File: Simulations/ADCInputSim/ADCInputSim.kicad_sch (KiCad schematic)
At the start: 8 parts, among them U1 ${SIM.PARAMS}

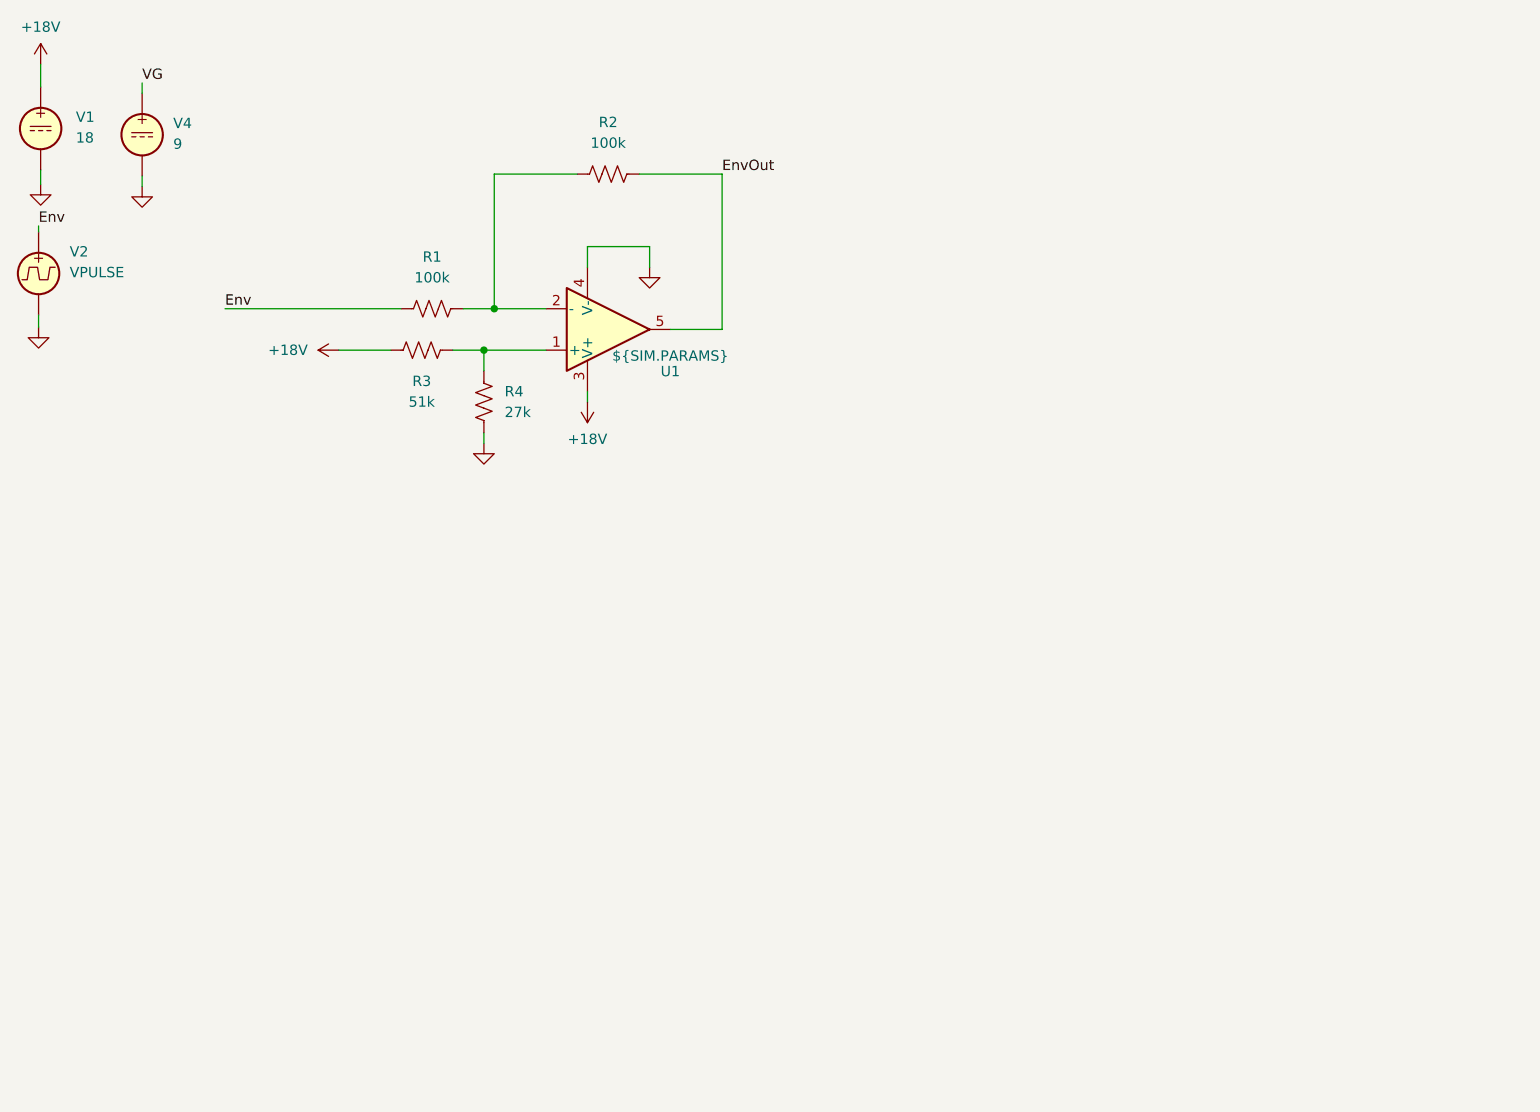
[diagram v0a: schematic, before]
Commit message: ADC driver dialed in
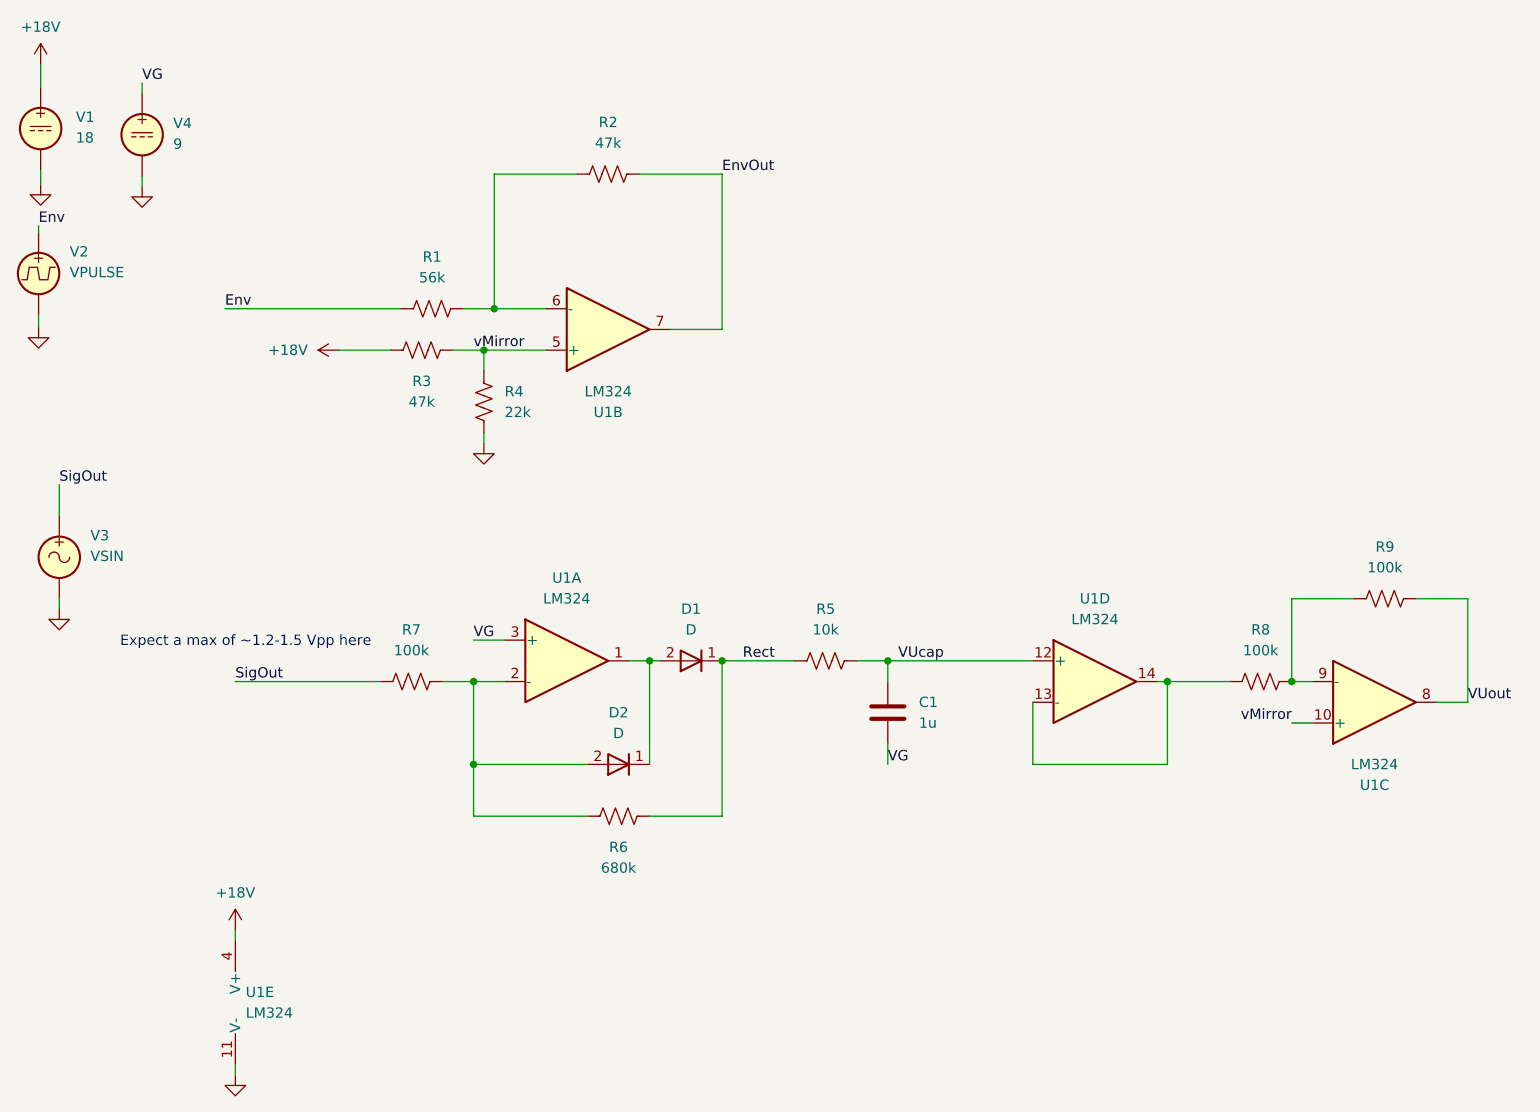
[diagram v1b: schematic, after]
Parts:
- removed U1: ${SIM.PARAMS}, symbol Simulation_SPICE:OPAMP
- added C1: 1u, symbol Device:C
- added D1, D2: D, symbol Simulation_SPICE:D
- added R5: 10k, symbol Device:R_US
- added R6: 680k, symbol Device:R_US
- added R7, R8, R9: 100k, symbol Device:R_US
- added U1: LM324, symbol Amplifier_Operational:LM324
- added V3: VSIN, symbol Simulation_SPICE:VSIN
- R1: value 100k -> 56k
- R2: value 100k -> 47k
- R3: value 51k -> 47k
- R4: value 27k -> 22k
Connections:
- net +18V: now also U1.4 (V+)
- net EnvOut: now also U1.7
- net GND: now also U1.11 (V-), V3.2
- net VG: now also C1.2, U1.3 (+)
- net vMirror: now reaches R3.2, R4.2
- net vMirror: now also U1.10 (+), U1.5 (+)
- net at R1.2, R2.1: now also U1.6 (-)
- new net: R8.1, U1.13 (-), U1.14
- new net: R8.2, R9.1, U1.9 (-)
- new net: D2.2 (A), R6.2, R7.1, U1.2 (-)
- new net: D1.2 (A), D2.1 (K), U1.1
- new net Rect: D1.1 (K), R5.1, R6.1
- new net SigOut: R7.2, V3.1
- new net VUcap: C1.1, R5.2, U1.12 (+)
- new net VUout: R9.2, U1.8
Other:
- note added: "Expect a max of ~1.2-1.5 Vpp here"
